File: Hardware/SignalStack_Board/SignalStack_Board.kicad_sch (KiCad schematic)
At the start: 74 parts, among them J2 RJ45_LED_Shielded, J3 Molex_uF_SV_06, Q1 SI4156DY, Q2 SI4156DY, Q3 SI4156DY, Q4 SI4156DY, Q5 SI4156DY, Q6 SI4156DY, Q7 SI4156DY, Q8 SI4156DY, Q9 Q_PMOS_DGS, SW1 SW_Push, SW2 SW_Push, U1 OKI, U10 74LVC2G04, U2 SMAJ12CA, U3 Teensy4.1_DEV-16771, U4 TSR_1-2450, U5 IRS2005S, U6 IRS2005S, U7 74LVC2G04, U8 IRS2005S, U9 IRS2005S

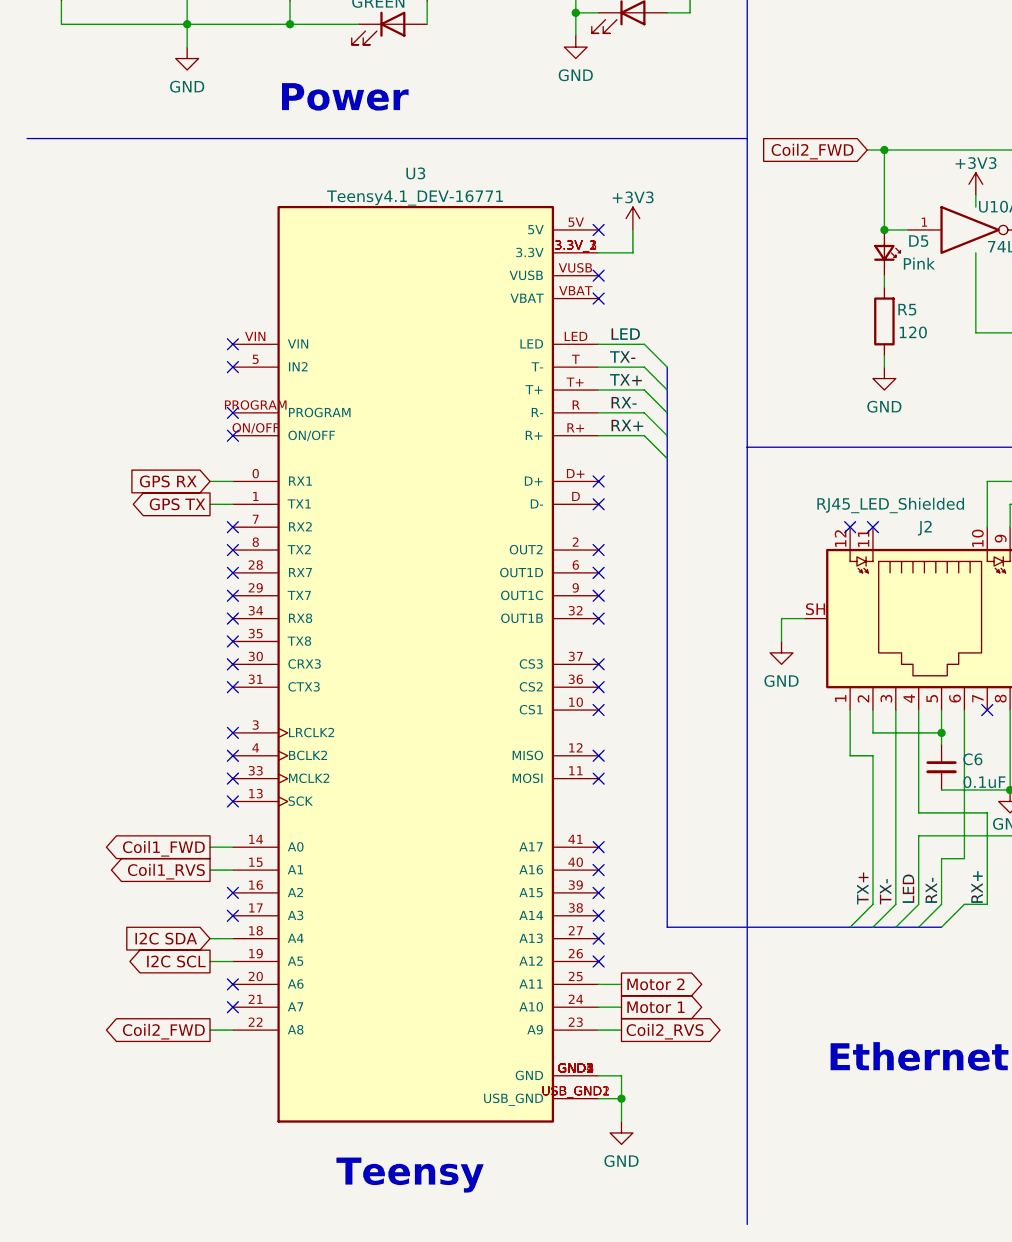
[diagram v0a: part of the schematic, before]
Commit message: Finished layout
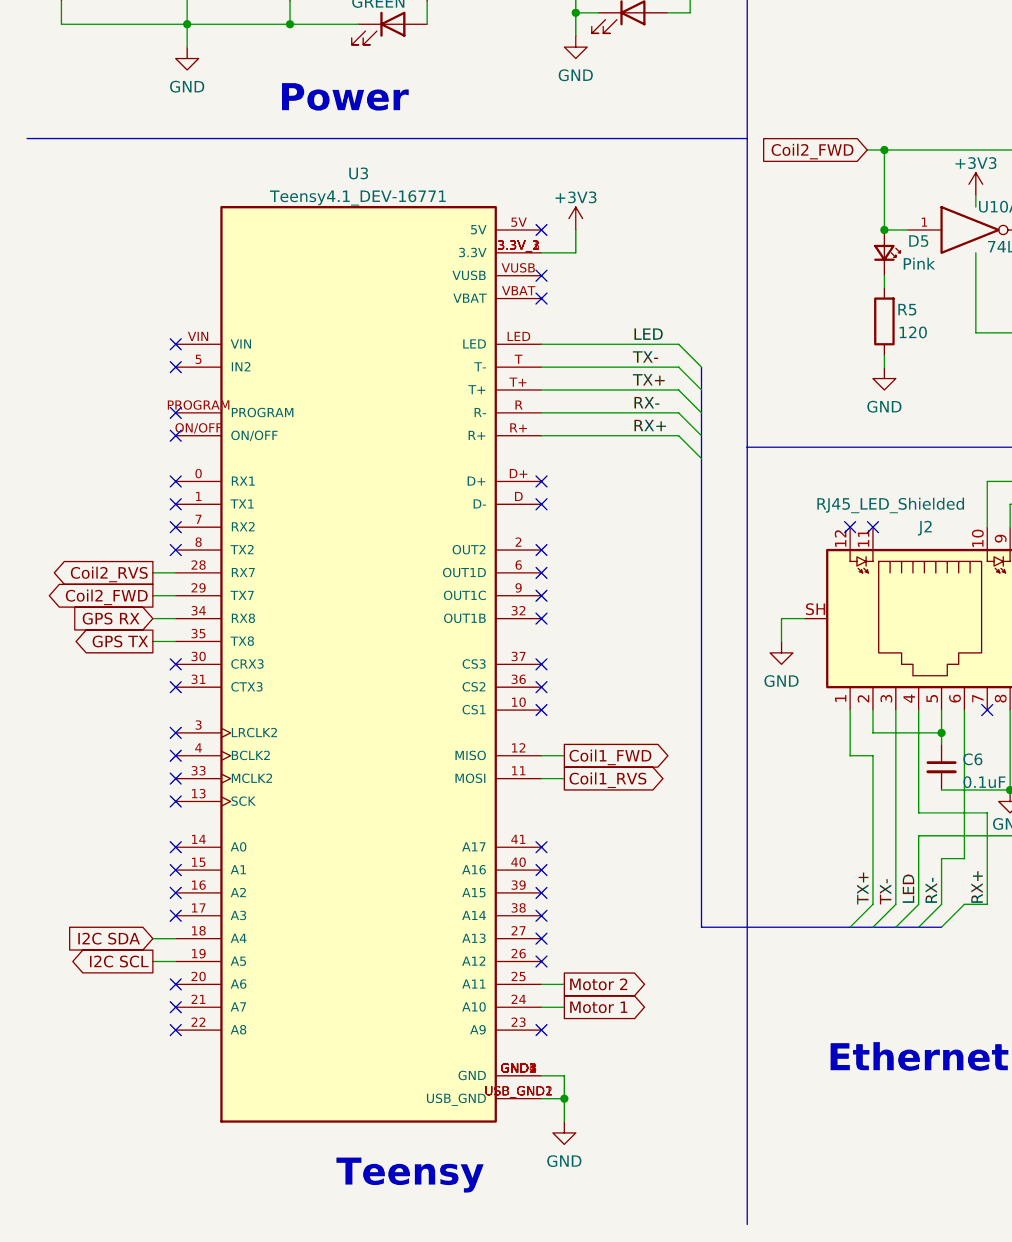
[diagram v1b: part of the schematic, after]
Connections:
- net Coil1_FWD: now also U3.12 (MISO); no longer U3.14 (A0)
- net Coil1_RVS: now also U3.11 (MOSI); no longer U3.15 (A1)
- net Coil2_FWD: now also U3.29 (TX7); no longer U3.22 (A8)
- net Coil2_RVS: now also U3.28 (RX7); no longer U3.23 (A9)
- net GPS RX: now also U3.34 (RX8); no longer U3.0 (RX1)
- net GPS TX: now also U3.35 (TX8); no longer U3.1 (TX1)
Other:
- moved on the sheet: U3
